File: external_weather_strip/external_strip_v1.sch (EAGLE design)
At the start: 11 parts, among them U1 ML8511-UV-SENSOR, U2 SHT21, U9 BMP180

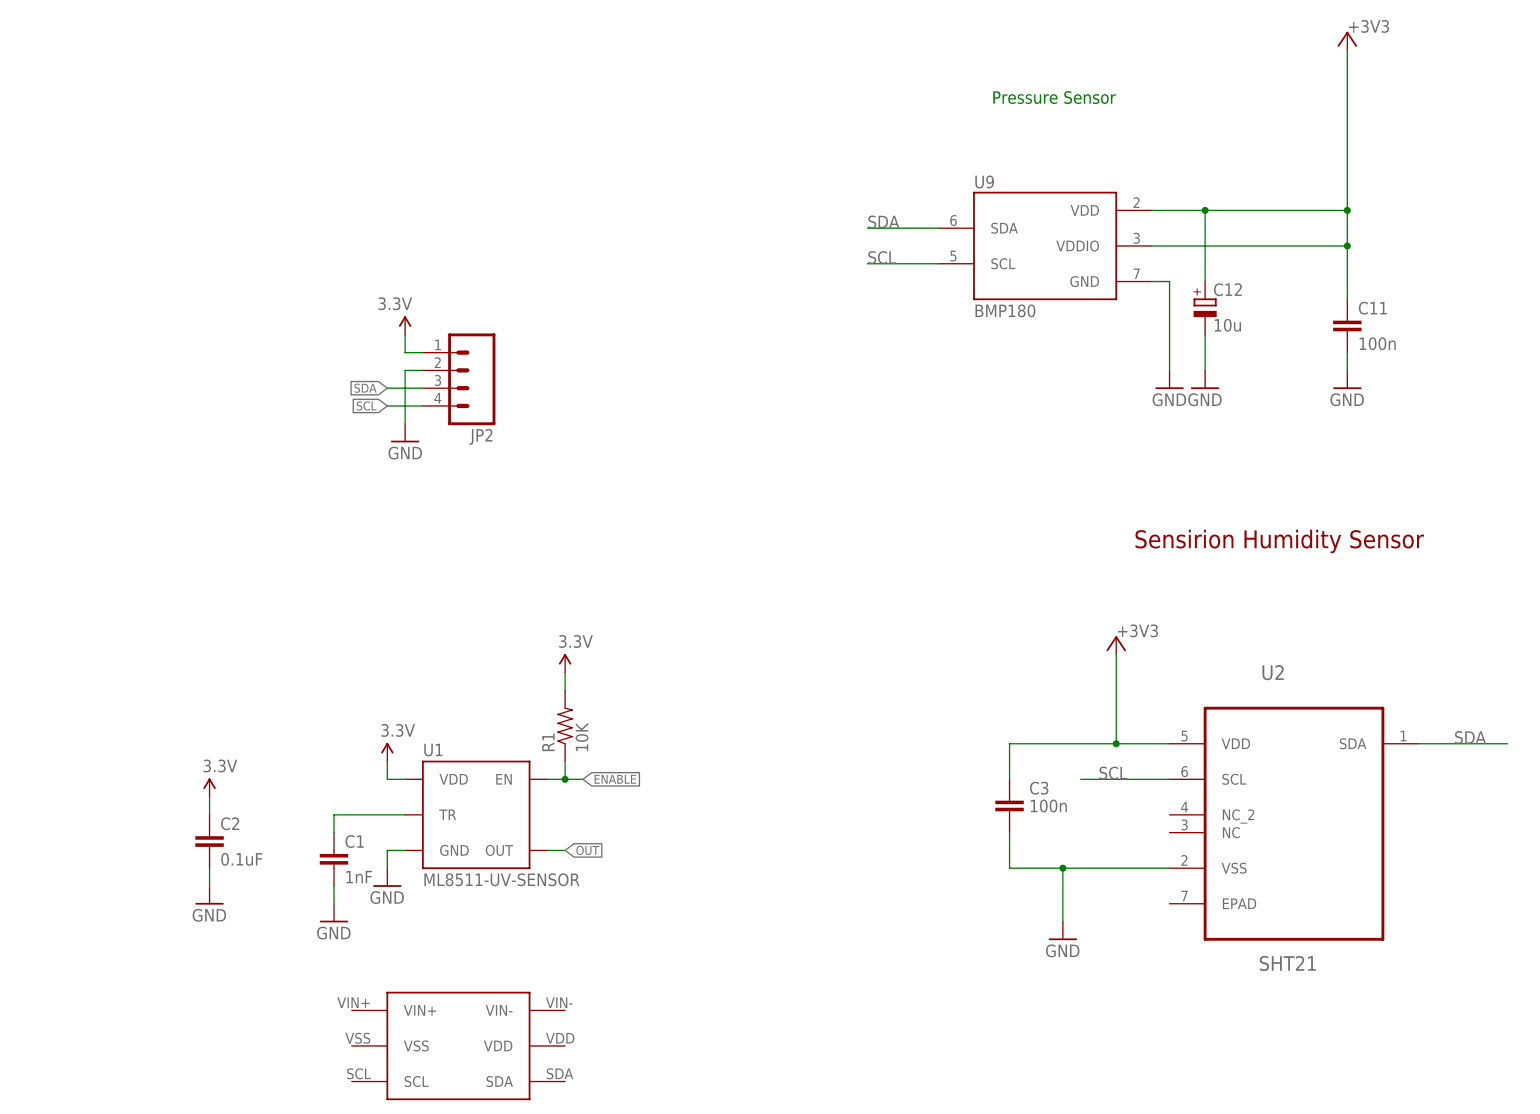
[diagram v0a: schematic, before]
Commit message: finished weather strip
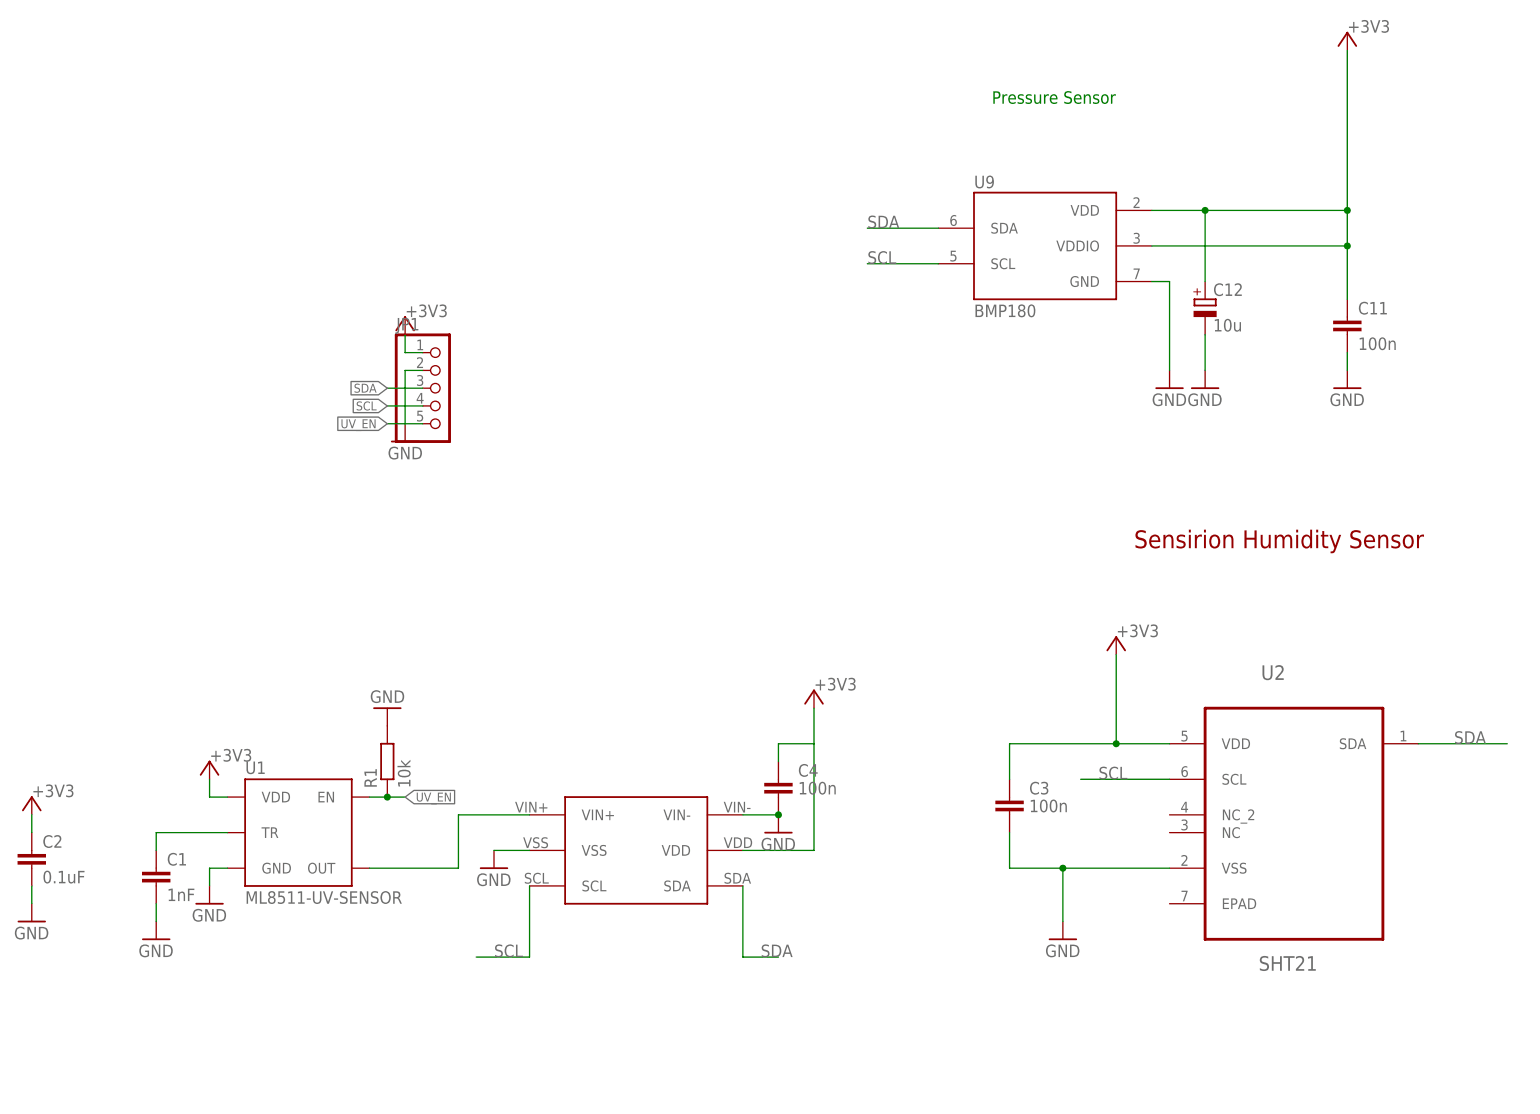
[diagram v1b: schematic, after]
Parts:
- removed JP2: (no value), SparkFun-Connectors:M04PTH
- added C4: 100n, rcl:C-EUC0603
- added JP1: (no value), Headerlibrary:PINHD-1X5
- R1: value 10K -> 10k; device SparkFun-Resistors:10KOHM1/10W1%(0603)0603 -> resistor:R-EU_R0603
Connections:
- removed net 3.3V: C2.1, JP2.1, R1.2, U1.VDD
- removed net ENABLE: R1.1, U1.EN
- removed net OUT: U1.OUT
- new net N$1: U$5.VIN+, U1.OUT
- new net UV_EN: JP1.5, R1.1, U1.EN
- net +3V3: now also C2.1, C4.1, JP1.1, U$5.VDD, U1.VDD
- net GND: now also C4.2, JP1.2, R1.2, U$5.VIN-, U$5.VSS; no longer JP2.2
- net SCL: now also JP1.4, U$5.SCL; no longer JP2.4
- net SDA: now also JP1.3, U$5.SDA; no longer JP2.3
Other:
- moved on the sheet: C1, C2, U1
